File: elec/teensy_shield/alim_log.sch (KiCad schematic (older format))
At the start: 0 parts

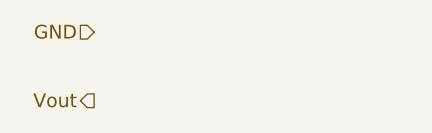
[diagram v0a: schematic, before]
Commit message: Completed new board schematics.
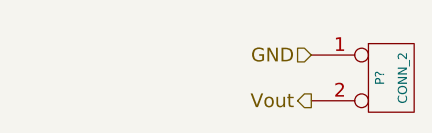
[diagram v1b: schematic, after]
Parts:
- added P?: CONN_2, symbol CONN_2
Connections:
- net GND: now also P?.1 (P1)
- net Vout: now also P?.2 (PM)
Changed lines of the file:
@@
 LIBS:contrib
 LIBS:valves
+LIBS:arduino_shieldsNCL
+LIBS:teensy
+LIBS:pololu
+LIBS:teensy_shield-cache
 EELAYER 24 0
 EELAYER END
 $Descr A4 11693 8268
 encoding utf-8
-Sheet 26 26
+Sheet 26 34
 Title ""
 Date ""
@@
 Comment4 ""
 $EndDescr
-Text HLabel 4100 2100 0    60   Input ~ 0
+Text HLabel 5050 2200 0    60   Input ~ 0
 GND
-Text HLabel 4100 2400 0    60   Output ~ 0
+Text HLabel 5050 2400 0    60   Output ~ 0
 Vout
+$Comp
+L CONN_2 P?
+U 1 1 55E8500F
+P 5400 2300
+F 0 "P?" V 5350 2300 40  0000 C CNN
+F 1 "CONN_2" V 5450 2300 40  0000 C CNN
+F 2 "" H 5400 2300 60  0000 C CNN
+F 3 "" H 5400 2300 60  0000 C CNN
+	1    5400 2300
+	1    0    0    -1
+$EndComp
 $EndSCHEMATC
